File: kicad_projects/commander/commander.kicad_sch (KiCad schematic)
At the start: 14 parts, among them J1 left input IDC14, J2 right input IDC14, J3 VIK FCC 12, J4 TPS pinout, J5 DS1020-12-6VBT1A-R, J6 PSP 3000 connector SFV4R-4STB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, J7 PSP 2000 raw pins out, J8 debug out, Q1 MMFTP3401, SW1 RESET_SWITCH, U1 Pico

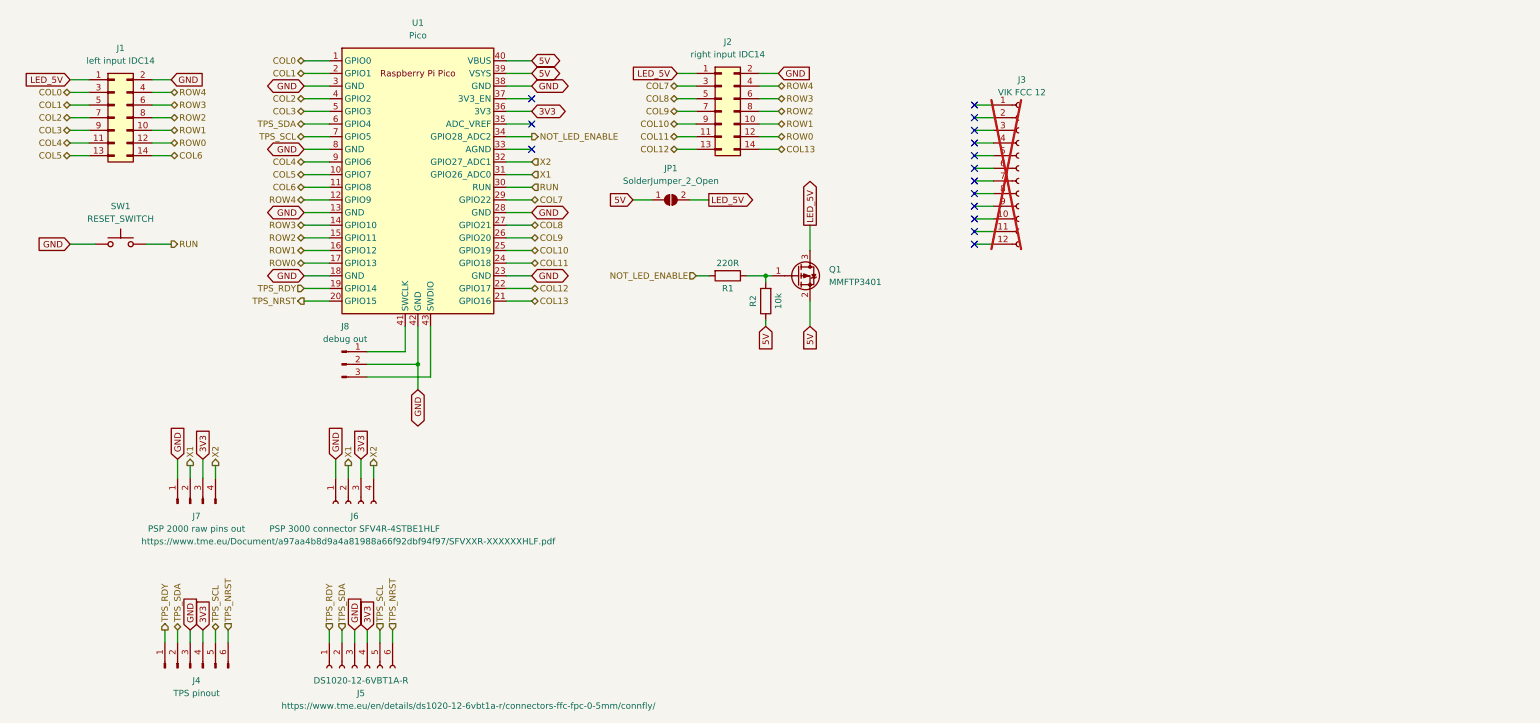
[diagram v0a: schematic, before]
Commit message: big commander WIP
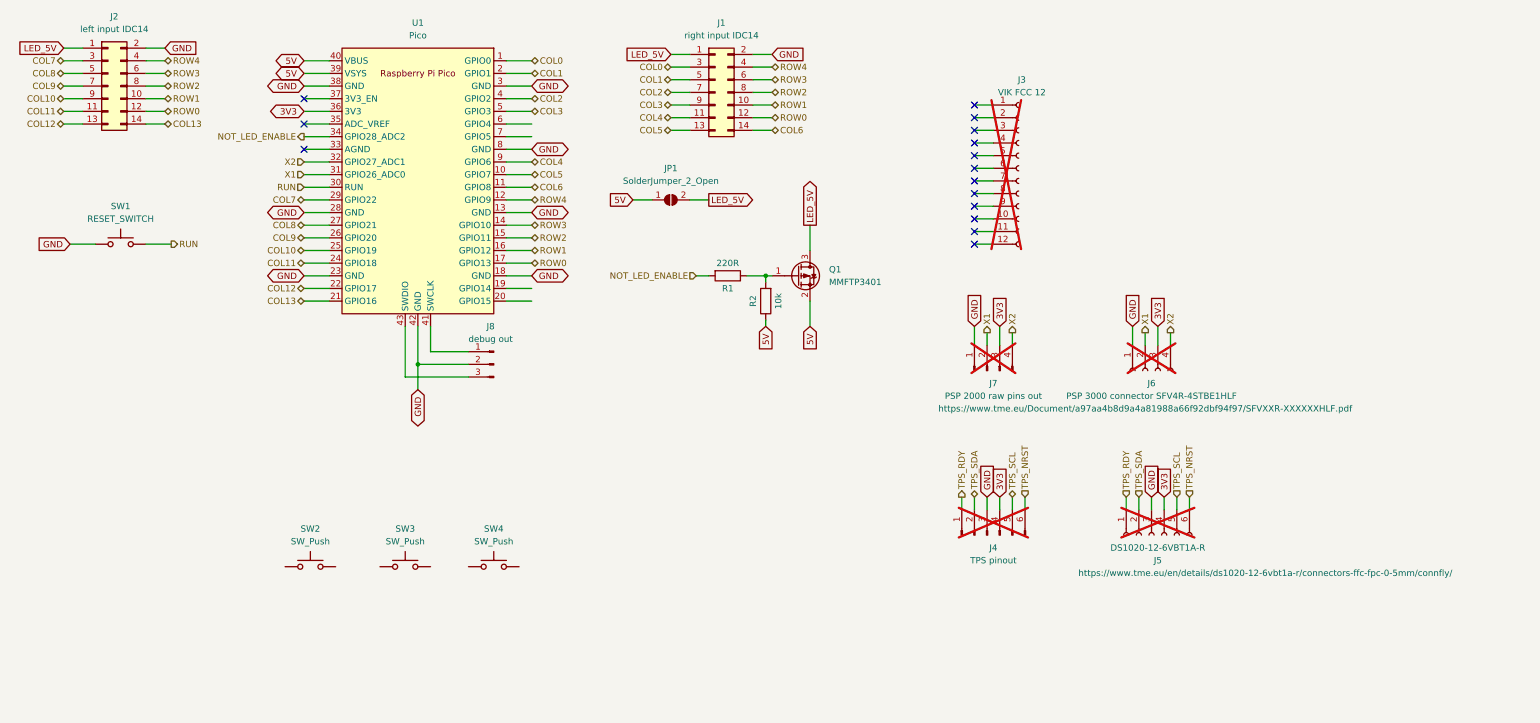
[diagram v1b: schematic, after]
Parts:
- added SW2, SW3, SW4: SW_Push, revolt_footprints:SW_PG1350_reversible_with_keycap_outline, symbol Switch:SW_Push
- J1: value left input IDC14 -> right input IDC14
- J2: value right input IDC14 -> left input IDC14
- J4, J5, J6, J7: now not fitted; now left out of the parts list
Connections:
- net TPS_NRST: no longer U1.20 (GPIO15)
- net TPS_RDY: no longer U1.19 (GPIO14)
- net TPS_SCL: no longer U1.7 (GPIO5)
- net TPS_SDA: no longer U1.6 (GPIO4)
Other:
- moved on the sheet: J1, J2, J8
